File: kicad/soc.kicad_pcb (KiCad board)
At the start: 2 copper layers, 104.1 x 63.5 mm, 40 parts, among them J1 Line Out, J2 PS/2 Keyboard, J3 Headphone Out, J4 Line In, P1 LED MATRIX, P2 ALTERA_DE1_GPIO, U1 SSM2603, U2 DS3234

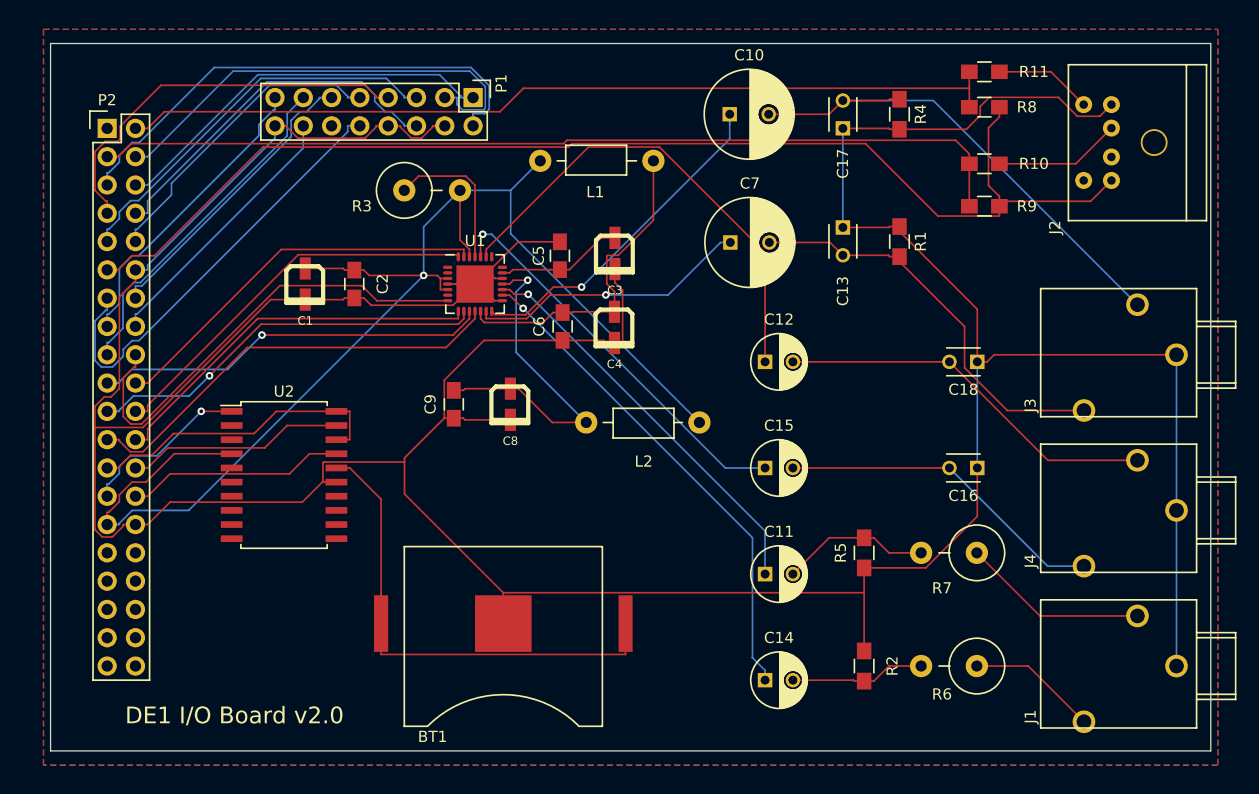
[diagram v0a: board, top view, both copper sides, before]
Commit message: start of IO board changes
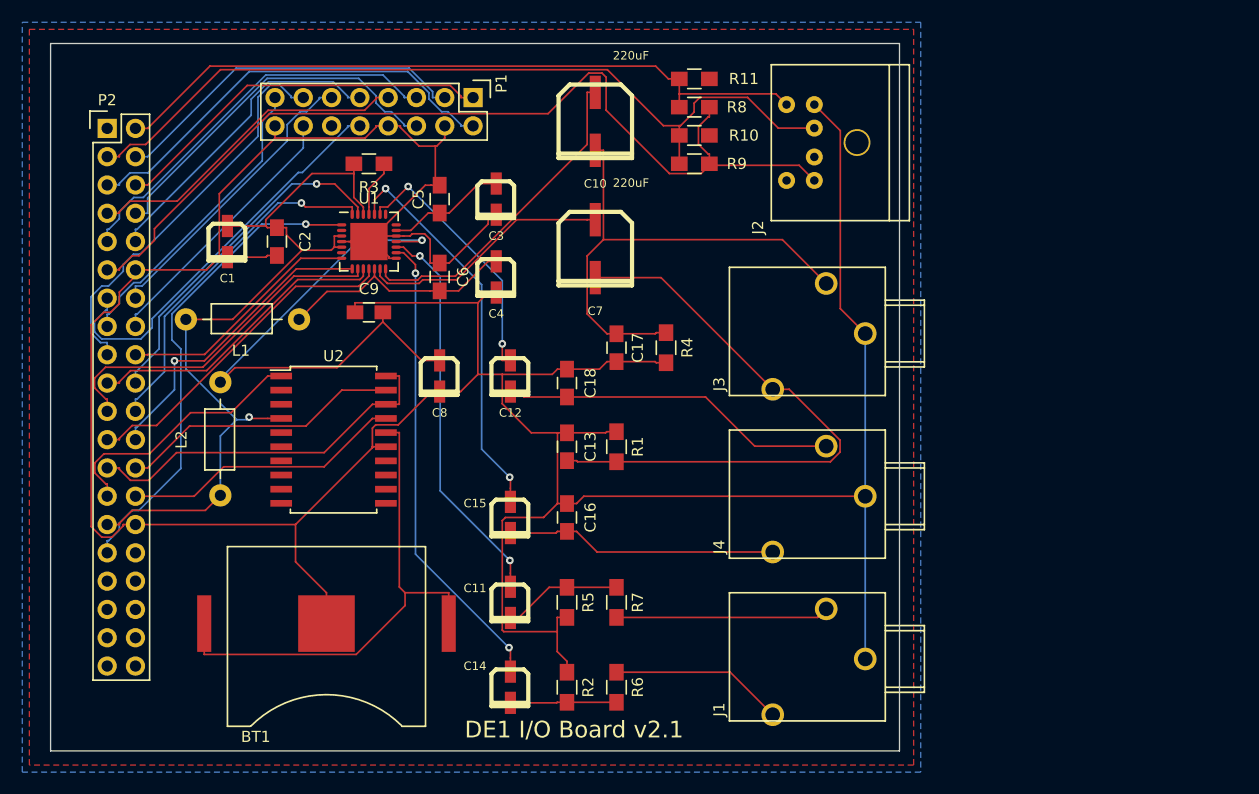
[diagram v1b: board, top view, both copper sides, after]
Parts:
- C10, C7: footprint Capacitors_ThroughHole:C_Radial_D8_L11.5_P3.5 -> mstock:UWXCAP-6.3mm
- C11, C12, C14, C15: footprint Capacitors_ThroughHole:C_Radial_D5_L6_P2.5 -> mstock:UWXCAP-3mm
- C13, C16, C17, C18: footprint Capacitors_ThroughHole:C_Disc_D3_P2.5 -> Capacitors_SMD:C_0805_HandSoldering
- R3, R6, R7: footprint Resistors_ThroughHole:Resistor_Vertical_RM5mm -> Resistors_SMD:R_0805_HandSoldering
- moved L2 38.0 mm to (55.9, 96.5), turned to 90 degrees
- moved C16 37.1 mm to (87.0, 103.5), turned to 270 degrees
- moved C18 36.9 mm to (87.0, 91.4), turned to 270 degrees
- moved L1 34.8 mm to (57.8, 85.7)
- moved C13 31.6 mm to (87.0, 97.2)
- moved R1 31.4 mm to (91.4, 97.2)
- moved R7 30.2 mm to (91.4, 111.1), turned to 90 degrees
- moved R6 29.9 mm to (91.4, 118.7), turned to 270 degrees
- moved R4 29.6 mm to (95.9, 88.3)
- moved C17 28.3 mm to (91.4, 88.3)
- moved J3 28.0 mm to (115.6, 87.0)
- moved J4 28.0 mm to (115.6, 101.6)
- moved J1 27.9 mm to (115.6, 116.2)
- moved R5 27.0 mm to (87.0, 111.1)
- moved R2 26.7 mm to (87.0, 118.7)
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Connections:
- J2 pad 1: Net-(J2-Pad1) -> /Kbd_data
- J2 pad 5: Net-(J2-Pad5) -> /Kbd_clk
- P2 pad 31: Net-(P2-Pad31) -> /MCLK
- U1 pad 1: Net-(U1-Pad1) -> /MCLK
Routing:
- net GND: track 376.6 -> 322.7 mm
- net +3V3: track 118.8 -> 75.1 mm
- net /MCLK: track 0.00 -> 43.6 mm, vias 0 -> 1
- net +5V: track 109.0 -> 84.0 mm
- net Net-(C12-Pad1): track 43.2 -> 23.8 mm, vias 0 -> 2
- net /BCLK: track 41.2 -> 22.1 mm
- net Net-(C8-Pad1): track 31.4 -> 50.2 mm
- net Net-(C13-Pad2): track 37.1 -> 54.0 mm
- net /Kbd_clk: track 79.5 -> 64.2 mm
- net Net-(J2-Pad1): track 11.4 -> 0.00 mm
- net /B0: track 41.6 -> 32.5 mm
- net /RECLRC: track 39.1 -> 30.3 mm
- net Net-(J2-Pad5): track 8.79 -> 0.00 mm
- net Net-(R3-Pad1): track 13.6 -> 5.09 mm
- net /Kbd_data: track 83.3 -> 75.0 mm
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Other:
- board size 104.1 x 63.5 mm -> 76.2 x 63.5 mm
- board text added: "DE1 I/O Board v2.1"
- board text removed: "DE1 I/O Board v2.0"
